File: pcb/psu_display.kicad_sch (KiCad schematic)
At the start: 9 parts, among them U1 TLV62568DBV

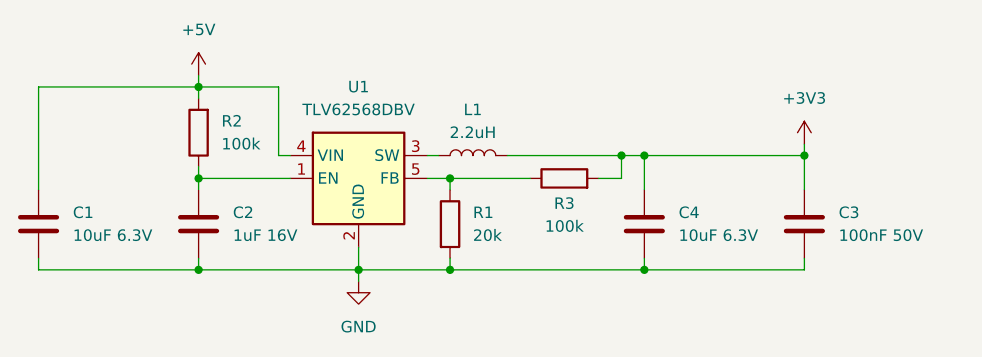
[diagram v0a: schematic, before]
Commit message: foo
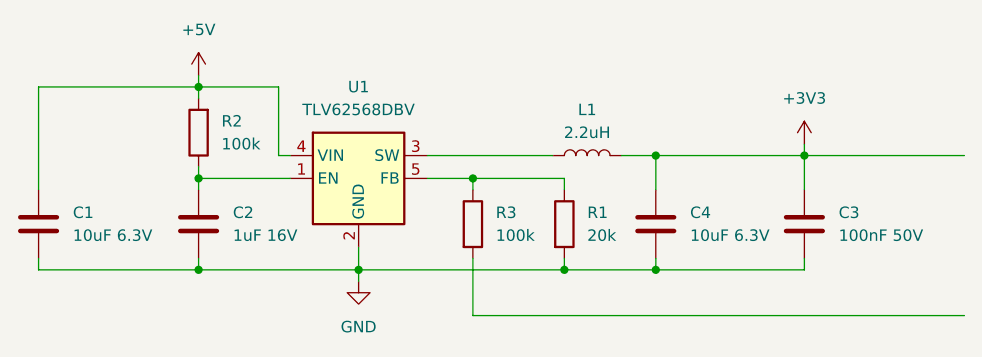
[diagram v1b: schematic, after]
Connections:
- net +3V3: no longer R3.2
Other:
- moved on the sheet: C4, L1, R1, R3
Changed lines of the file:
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@@
 	(paper "A4")
 	(junction
-		(at 95.25 58.42)
-		(diameter 0)
-		(color 0 0 0 0)
-	)
-	(junction
-		(at 116.84 68.58)
-		(diameter 0)
-		(color 0 0 0 0)
-	)
-	(junction
-		(at 114.3 55.88)
+		(at 107.95 68.58)
 		(diameter 0)
 		(color 0 0 0 0)
@@
 	)
 	(junction
-		(at 116.84 55.88)
+		(at 118.11 68.58)
+		(diameter 0)
+		(color 0 0 0 0)
+	)
+	(junction
+		(at 118.11 55.88)
 		(diameter 0)
 		(color 0 0 0 0)
@@
 	)
 	(junction
-		(at 67.31 48.26)
+		(at 97.79 58.42)
 		(diameter 0)
 		(color 0 0 0 0)
 	)
 	(junction
-		(at 95.25 68.58)
+		(at 67.31 48.26)
 		(diameter 0)
 		(color 0 0 0 0)
@@
 	(wire
 		(pts
-			(xy 111.76 58.42) (xy 114.3 58.42)
-		)
-		(stroke
-			(width 0)
-			(type default)
-		)
-	)
-	(wire
-		(pts
 			(xy 76.2 48.26) (xy 76.2 55.88)
 		)
@@
 	(wire
 		(pts
-			(xy 114.3 58.42) (xy 114.3 55.88)
-		)
-		(stroke
-			(width 0)
-			(type default)
-		)
-	)
-	(wire
-		(pts
-			(xy 116.84 67.31) (xy 116.84 68.58)
-		)
-		(stroke
-			(width 0)
-			(type default)
-		)
-	)
-	(wire
-		(pts
-			(xy 95.25 58.42) (xy 104.14 58.42)
-		)
-		(stroke
-			(width 0)
-			(type default)
-		)
-	)
-	(wire
-		(pts
-			(xy 95.25 67.31) (xy 95.25 68.58)
-		)
-		(stroke
-			(width 0)
-			(type default)
-		)
-	)
-	(wire
-		(pts
-			(xy 92.71 58.42) (xy 95.25 58.42)
+			(xy 97.79 58.42) (xy 97.79 59.69)
+		)
+		(stroke
+			(width 0)
+			(type default)
+		)
+	)
+	(wire
+		(pts
+			(xy 97.79 58.42) (xy 107.95 58.42)
+		)
+		(stroke
+			(width 0)
+			(type default)
+		)
+	)
+	(wire
+		(pts
+			(xy 118.11 67.31) (xy 118.11 68.58)
+		)
+		(stroke
+			(width 0)
+			(type default)
+		)
+	)
+	(wire
+		(pts
+			(xy 134.62 68.58) (xy 118.11 68.58)
+		)
+		(stroke
+			(width 0)
+			(type default)
+		)
+	)
+	(wire
+		(pts
+			(xy 107.95 67.31) (xy 107.95 68.58)
+		)
+		(stroke
+			(width 0)
+			(type default)
+		)
+	)
+	(wire
+		(pts
+			(xy 92.71 58.42) (xy 97.79 58.42)
 		)
 		(stroke
@@
 	(wire
 		(pts
-			(xy 92.71 55.88) (xy 93.98 55.88)
-		)
-		(stroke
-			(width 0)
-			(type default)
-		)
-	)
-	(wire
-		(pts
-			(xy 95.25 68.58) (xy 85.09 68.58)
+			(xy 92.71 55.88) (xy 106.68 55.88)
+		)
+		(stroke
+			(width 0)
+			(type default)
+		)
+	)
+	(wire
+		(pts
+			(xy 107.95 68.58) (xy 85.09 68.58)
 		)
 		(stroke
@@
 	(wire
 		(pts
-			(xy 116.84 55.88) (xy 134.62 55.88)
-		)
-		(stroke
-			(width 0)
-			(type default)
-		)
-	)
-	(wire
-		(pts
-			(xy 95.25 58.42) (xy 95.25 59.69)
+			(xy 134.62 55.88) (xy 152.4 55.88)
+		)
+		(stroke
+			(width 0)
+			(type default)
+		)
+	)
+	(wire
+		(pts
+			(xy 107.95 58.42) (xy 107.95 59.69)
 		)
 		(stroke
@@
 	(wire
 		(pts
-			(xy 95.25 68.58) (xy 116.84 68.58)
-		)
-		(stroke
-			(width 0)
-			(type default)
-		)
-	)
-	(wire
-		(pts
 			(xy 85.09 68.58) (xy 85.09 69.85)
 		)
@@
 	(wire
 		(pts
+			(xy 118.11 55.88) (xy 134.62 55.88)
+		)
+		(stroke
+			(width 0)
+			(type default)
+		)
+	)
+	(wire
+		(pts
 			(xy 134.62 59.69) (xy 134.62 55.88)
 		)
@@
 	(wire
 		(pts
-			(xy 101.6 55.88) (xy 114.3 55.88)
+			(xy 114.3 55.88) (xy 118.11 55.88)
 		)
 		(stroke
@@
 	(wire
 		(pts
-			(xy 114.3 55.88) (xy 116.84 55.88)
-		)
-		(stroke
-			(width 0)
-			(type default)
-		)
-	)
-	(wire
-		(pts
-			(xy 116.84 59.69) (xy 116.84 55.88)
+			(xy 118.11 59.69) (xy 118.11 55.88)
+		)
+		(stroke
+			(width 0)
+			(type default)
+		)
+	)
+	(wire
+		(pts
+			(xy 97.79 67.31) (xy 97.79 73.66)
 		)
 		(stroke
@@
 	(wire
 		(pts
-			(xy 116.84 68.58) (xy 134.62 68.58)
-		)
-		(stroke
-			(width 0)
-			(type default)
-		)
-	)
-	(wire
-		(pts
 			(xy 67.31 46.99) (xy 67.31 48.26)
+		)
+		(stroke
+			(width 0)
+			(type default)
+		)
+	)
+	(wire
+		(pts
+			(xy 118.11 68.58) (xy 107.95 68.58)
+		)
+		(stroke
+			(width 0)
+			(type default)
+		)
+	)
+	(wire
+		(pts
+			(xy 97.79 73.66) (xy 152.4 73.66)
 		)
 		(stroke
@@
 	(symbol
 		(lib_id "Device:L")
-		(at 97.79 55.88 90)
+		(at 110.49 55.88 90)
 		(unit 1)
 		(exclude_from_sim no)
@@
 		(on_board yes)
 		(dnp no)
+		(fields_autoplaced yes)
 		(property "Reference" "L1"
-			(at 97.79 50.8 90)
+			(at 110.49 50.8 90)
 			(effects
 				(font
@@
 		)
 		(property "Value" "2.2uH"
-			(at 97.79 53.34 90)
+			(at 110.49 53.34 90)
 			(effects
 				(font
@@
 		)
 		(property "Footprint" "Inductor_SMD:L_Bourns-SRN4018"
-			(at 97.79 55.88 0)
+			(at 110.49 55.88 0)
 			(effects
 				(font
@@
 		)
 		(property "Datasheet" "~"
-			(at 97.79 55.88 0)
+			(at 110.49 55.88 0)
 			(effects
 				(font
@@
 		)
 		(property "Description" "Inductor"
-			(at 97.79 55.88 0)
+			(at 110.49 55.88 0)
 			(effects
 				(font
@@
 	(symbol
 		(lib_id "Device:C")
-		(at 116.84 63.5 0)
+		(at 118.11 63.5 0)
 		(unit 1)
 		(exclude_from_sim no)
@@
 		(fields_autoplaced yes)
 		(property "Reference" "C4"
-			(at 120.65 62.2299 0)
+			(at 121.92 62.2299 0)
 			(effects
 				(font
@@
 		)
 		(property "Value" "10uF 6.3V"
-			(at 120.65 64.7699 0)
+			(at 121.92 64.7699 0)
 			(effects
 				(font
@@
 		)
 		(property "Footprint" "Capacitor_SMD:C_0805_2012Metric_Pad1.18x1.45mm_HandSolder"
-			(at 117.8052 67.31 0)
+			(at 119.0752 67.31 0)
 			(effects
 				(font
@@
 		)
 		(property "Datasheet" "~"
-			(at 116.84 63.5 0)
+			(at 118.11 63.5 0)
 			(effects
 				(font
@@
 		)
 		(property "Description" "Unpolarized capacitor"
-			(at 116.84 63.5 0)
+			(at 118.11 63.5 0)
 			(effects
 				(font
@@
 	(symbol
 		(lib_id "Device:R")
-		(at 95.25 63.5 0)
+		(at 107.95 63.5 0)
 		(unit 1)
 		(exclude_from_sim no)
@@
 		(fields_autoplaced yes)
 		(property "Reference" "R1"
-			(at 97.79 62.2299 0)
+			(at 110.49 62.2299 0)
 			(effects
 				(font
@@
 		)
 		(property "Value" "20k"
-			(at 97.79 64.7699 0)
+			(at 110.49 64.7699 0)
 			(effects
 				(font
@@
 		)
 		(property "Footprint" "Resistor_SMD:R_0603_1608Metric_Pad0.98x0.95mm_HandSolder"
-			(at 93.472 63.5 90)
+			(at 106.172 63.5 90)
 			(effects
 				(font
@@
 		)
 		(property "Datasheet" "~"
-			(at 95.25 63.5 0)
+			(at 107.95 63.5 0)
 			(effects
 				(font
@@
 		)
 		(property "Description" "Resistor"
-			(at 95.25 63.5 0)
+			(at 107.95 63.5 0)
 			(effects
 				(font
@@
 	(symbol
 		(lib_id "Device:R")
-		(at 107.95 58.42 90)
+		(at 97.79 63.5 0)
 		(unit 1)
 		(exclude_from_sim no)
@@
 		(on_board yes)
 		(dnp no)
+		(fields_autoplaced yes)
 		(property "Reference" "R3"
-			(at 107.95 61.214 90)
-			(effects
-				(font
-					(size 1.27 1.27)
-				)
+			(at 100.33 62.2299 0)
+			(effects
+				(font
+					(size 1.27 1.27)
+				)
+				(justify left)
 			)
 		)
 		(property "Value" "100k"
-			(at 107.95 63.754 90)
-			(effects
-				(font
-					(size 1.27 1.27)
-				)
+			(at 100.33 64.7699 0)
+			(effects
+				(font
+					(size 1.27 1.27)
+				)
+				(justify left)
 			)
 		)
 		(property "Footprint" "Resistor_SMD:R_0603_1608Metric_Pad0.98x0.95mm_HandSolder"
-			(at 107.95 60.198 90)
+			(at 96.012 63.5 90)
 			(effects
 				(font
@@
 		)
 		(property "Datasheet" "~"
-			(at 107.95 58.42 0)
+			(at 97.79 63.5 0)
 			(effects
 				(font
@@
 		)
 		(property "Description" "Resistor"
-			(at 107.95 58.42 0)
-			(effects
-				(font
+			(at 97.79 63.5 0)
+			(effects
+				(font

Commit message: display connections done
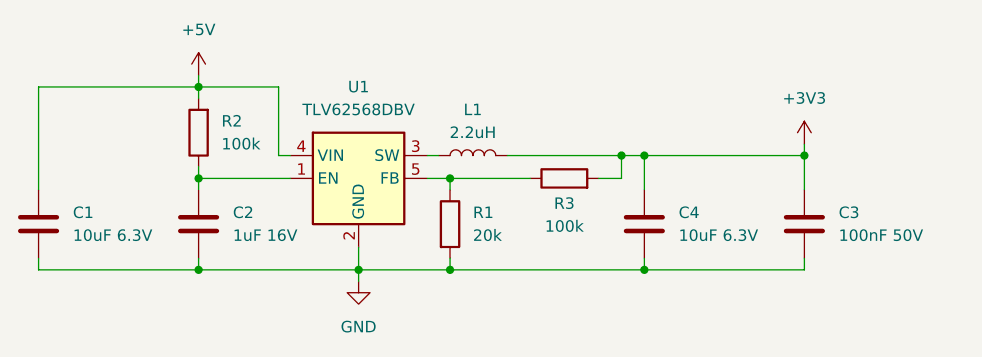
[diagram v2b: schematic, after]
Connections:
- net +3V3: now also R3.2
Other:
- moved on the sheet: C4, L1, R1, R3
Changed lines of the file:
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@@
 	(paper "A4")
 	(junction
-		(at 107.95 68.58)
+		(at 95.25 58.42)
+		(diameter 0)
+		(color 0 0 0 0)
+	)
+	(junction
+		(at 116.84 68.58)
+		(diameter 0)
+		(color 0 0 0 0)
+	)
+	(junction
+		(at 114.3 55.88)
 		(diameter 0)
 		(color 0 0 0 0)
@@
 	)
 	(junction
-		(at 118.11 68.58)
-		(diameter 0)
-		(color 0 0 0 0)
-	)
-	(junction
-		(at 118.11 55.88)
+		(at 116.84 55.88)
 		(diameter 0)
 		(color 0 0 0 0)
@@
 	)
 	(junction
-		(at 97.79 58.42)
+		(at 67.31 48.26)
 		(diameter 0)
 		(color 0 0 0 0)
 	)
 	(junction
-		(at 67.31 48.26)
+		(at 95.25 68.58)
 		(diameter 0)
 		(color 0 0 0 0)
@@
 	(wire
 		(pts
+			(xy 111.76 58.42) (xy 114.3 58.42)
+		)
+		(stroke
+			(width 0)
+			(type default)
+		)
+	)
+	(wire
+		(pts
 			(xy 76.2 48.26) (xy 76.2 55.88)
 		)
@@
 	(wire
 		(pts
-			(xy 97.79 58.42) (xy 97.79 59.69)
-		)
-		(stroke
-			(width 0)
-			(type default)
-		)
-	)
-	(wire
-		(pts
-			(xy 97.79 58.42) (xy 107.95 58.42)
-		)
-		(stroke
-			(width 0)
-			(type default)
-		)
-	)
-	(wire
-		(pts
-			(xy 118.11 67.31) (xy 118.11 68.58)
-		)
-		(stroke
-			(width 0)
-			(type default)
-		)
-	)
-	(wire
-		(pts
-			(xy 134.62 68.58) (xy 118.11 68.58)
-		)
-		(stroke
-			(width 0)
-			(type default)
-		)
-	)
-	(wire
-		(pts
-			(xy 107.95 67.31) (xy 107.95 68.58)
-		)
-		(stroke
-			(width 0)
-			(type default)
-		)
-	)
-	(wire
-		(pts
-			(xy 92.71 58.42) (xy 97.79 58.42)
+			(xy 114.3 58.42) (xy 114.3 55.88)
+		)
+		(stroke
+			(width 0)
+			(type default)
+		)
+	)
+	(wire
+		(pts
+			(xy 116.84 67.31) (xy 116.84 68.58)
+		)
+		(stroke
+			(width 0)
+			(type default)
+		)
+	)
+	(wire
+		(pts
+			(xy 95.25 58.42) (xy 104.14 58.42)
+		)
+		(stroke
+			(width 0)
+			(type default)
+		)
+	)
+	(wire
+		(pts
+			(xy 95.25 67.31) (xy 95.25 68.58)
+		)
+		(stroke
+			(width 0)
+			(type default)
+		)
+	)
+	(wire
+		(pts
+			(xy 92.71 58.42) (xy 95.25 58.42)
 		)
 		(stroke
@@
 	(wire
 		(pts
-			(xy 92.71 55.88) (xy 106.68 55.88)
-		)
-		(stroke
-			(width 0)
-			(type default)
-		)
-	)
-	(wire
-		(pts
-			(xy 107.95 68.58) (xy 85.09 68.58)
+			(xy 92.71 55.88) (xy 93.98 55.88)
+		)
+		(stroke
+			(width 0)
+			(type default)
+		)
+	)
+	(wire
+		(pts
+			(xy 95.25 68.58) (xy 85.09 68.58)
 		)
 		(stroke
@@
 	(wire
 		(pts
-			(xy 134.62 55.88) (xy 152.4 55.88)
-		)
-		(stroke
-			(width 0)
-			(type default)
-		)
-	)
-	(wire
-		(pts
-			(xy 107.95 58.42) (xy 107.95 59.69)
+			(xy 116.84 55.88) (xy 134.62 55.88)
+		)
+		(stroke
+			(width 0)
+			(type default)
+		)
+	)
+	(wire
+		(pts
+			(xy 95.25 58.42) (xy 95.25 59.69)
 		)
 		(stroke
@@
 	(wire
 		(pts
+			(xy 95.25 68.58) (xy 116.84 68.58)
+		)
+		(stroke
+			(width 0)
+			(type default)
+		)
+	)
+	(wire
+		(pts
 			(xy 85.09 68.58) (xy 85.09 69.85)
 		)
@@
 	(wire
 		(pts
-			(xy 118.11 55.88) (xy 134.62 55.88)
-		)
-		(stroke
-			(width 0)
-			(type default)
-		)
-	)
-	(wire
-		(pts
 			(xy 134.62 59.69) (xy 134.62 55.88)
 		)
@@
 	(wire
 		(pts
-			(xy 114.3 55.88) (xy 118.11 55.88)
+			(xy 101.6 55.88) (xy 114.3 55.88)
 		)
 		(stroke
@@
 	(wire
 		(pts
-			(xy 118.11 59.69) (xy 118.11 55.88)
-		)
-		(stroke
-			(width 0)
-			(type default)
-		)
-	)
-	(wire
-		(pts
-			(xy 97.79 67.31) (xy 97.79 73.66)
+			(xy 114.3 55.88) (xy 116.84 55.88)
+		)
+		(stroke
+			(width 0)
+			(type default)
+		)
+	)
+	(wire
+		(pts
+			(xy 116.84 59.69) (xy 116.84 55.88)
 		)
 		(stroke
@@
 	(wire
 		(pts
+			(xy 116.84 68.58) (xy 134.62 68.58)
+		)
+		(stroke
+			(width 0)
+			(type default)
+		)
+	)
+	(wire
+		(pts
 			(xy 67.31 46.99) (xy 67.31 48.26)
-		)
-		(stroke
-			(width 0)
-			(type default)
-		)
-	)
-	(wire
-		(pts
-			(xy 118.11 68.58) (xy 107.95 68.58)
-		)
-		(stroke
-			(width 0)
-			(type default)
-		)
-	)
-	(wire
-		(pts
-			(xy 97.79 73.66) (xy 152.4 73.66)
 		)
 		(stroke
@@
 	(symbol
 		(lib_id "Device:L")
-		(at 110.49 55.88 90)
+		(at 97.79 55.88 90)
 		(unit 1)
 		(exclude_from_sim no)
@@
 		(on_board yes)
 		(dnp no)
-		(fields_autoplaced yes)
 		(property "Reference" "L1"
-			(at 110.49 50.8 90)
+			(at 97.79 50.8 90)
 			(effects
 				(font
@@
 		)
 		(property "Value" "2.2uH"
-			(at 110.49 53.34 90)
+			(at 97.79 53.34 90)
 			(effects
 				(font
@@
 		)
 		(property "Footprint" "Inductor_SMD:L_Bourns-SRN4018"
-			(at 110.49 55.88 0)
+			(at 97.79 55.88 0)
 			(effects
 				(font
@@
 		)
 		(property "Datasheet" "~"
-			(at 110.49 55.88 0)
+			(at 97.79 55.88 0)
 			(effects
 				(font
@@
 		)
 		(property "Description" "Inductor"
-			(at 110.49 55.88 0)
+			(at 97.79 55.88 0)
 			(effects
 				(font
@@
 	(symbol
 		(lib_id "Device:C")
-		(at 118.11 63.5 0)
+		(at 116.84 63.5 0)
 		(unit 1)
 		(exclude_from_sim no)
@@
 		(fields_autoplaced yes)
 		(property "Reference" "C4"
-			(at 121.92 62.2299 0)
+			(at 120.65 62.2299 0)
 			(effects
 				(font
@@
 		)
 		(property "Value" "10uF 6.3V"
-			(at 121.92 64.7699 0)
+			(at 120.65 64.7699 0)
 			(effects
 				(font
@@
 		)
 		(property "Footprint" "Capacitor_SMD:C_0805_2012Metric_Pad1.18x1.45mm_HandSolder"
-			(at 119.0752 67.31 0)
+			(at 117.8052 67.31 0)
 			(effects
 				(font
@@
 		)
 		(property "Datasheet" "~"
-			(at 118.11 63.5 0)
+			(at 116.84 63.5 0)
 			(effects
 				(font
@@
 		)
 		(property "Description" "Unpolarized capacitor"
-			(at 118.11 63.5 0)
+			(at 116.84 63.5 0)
 			(effects
 				(font
@@
 	(symbol
 		(lib_id "Device:R")
-		(at 107.95 63.5 0)
+		(at 95.25 63.5 0)
 		(unit 1)
 		(exclude_from_sim no)
@@
 		(fields_autoplaced yes)
 		(property "Reference" "R1"
-			(at 110.49 62.2299 0)
+			(at 97.79 62.2299 0)
 			(effects
 				(font
@@
 		)
 		(property "Value" "20k"
-			(at 110.49 64.7699 0)
+			(at 97.79 64.7699 0)
 			(effects
 				(font
@@
 		)
 		(property "Footprint" "Resistor_SMD:R_0603_1608Metric_Pad0.98x0.95mm_HandSolder"
-			(at 106.172 63.5 90)
+			(at 93.472 63.5 90)
 			(effects
 				(font
@@
 		)
 		(property "Datasheet" "~"
-			(at 107.95 63.5 0)
+			(at 95.25 63.5 0)
 			(effects
 				(font
@@
 		)
 		(property "Description" "Resistor"
-			(at 107.95 63.5 0)
+			(at 95.25 63.5 0)
 			(effects
 				(font
@@
 	(symbol
 		(lib_id "Device:R")
-		(at 97.79 63.5 0)
+		(at 107.95 58.42 90)
 		(unit 1)
 		(exclude_from_sim no)
@@
 		(on_board yes)
 		(dnp no)
-		(fields_autoplaced yes)
 		(property "Reference" "R3"
-			(at 100.33 62.2299 0)
-			(effects
-				(font
-					(size 1.27 1.27)
-				)
-				(justify left)
+			(at 107.95 61.214 90)
+			(effects
+				(font
+					(size 1.27 1.27)
+				)
 			)
 		)
 		(property "Value" "100k"
-			(at 100.33 64.7699 0)
-			(effects
-				(font
-					(size 1.27 1.27)
-				)
-				(justify left)
+			(at 107.95 63.754 90)
+			(effects
+				(font
+					(size 1.27 1.27)
+				)
 			)
 		)
 		(property "Footprint" "Resistor_SMD:R_0603_1608Metric_Pad0.98x0.95mm_HandSolder"
-			(at 96.012 63.5 90)
+			(at 107.95 60.198 90)
 			(effects
 				(font
@@
 		)
 		(property "Datasheet" "~"
-			(at 97.79 63.5 0)
+			(at 107.95 58.42 0)
 			(effects
 				(font
@@
 		)
 		(property "Description" "Resistor"
-			(at 97.79 63.5 0)
-			(effects
-				(font
+			(at 107.95 58.42 0)
+			(effects
+				(font
